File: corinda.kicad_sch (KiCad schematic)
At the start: 15 parts, among them J1 Pixels, J2 USB_B_Micro, J3 ExtPwr, J4 ExtPwr2, SW1 RESET, U1 ME6211, U2 ESP-C3-13U, U3 D1_Mini_16p

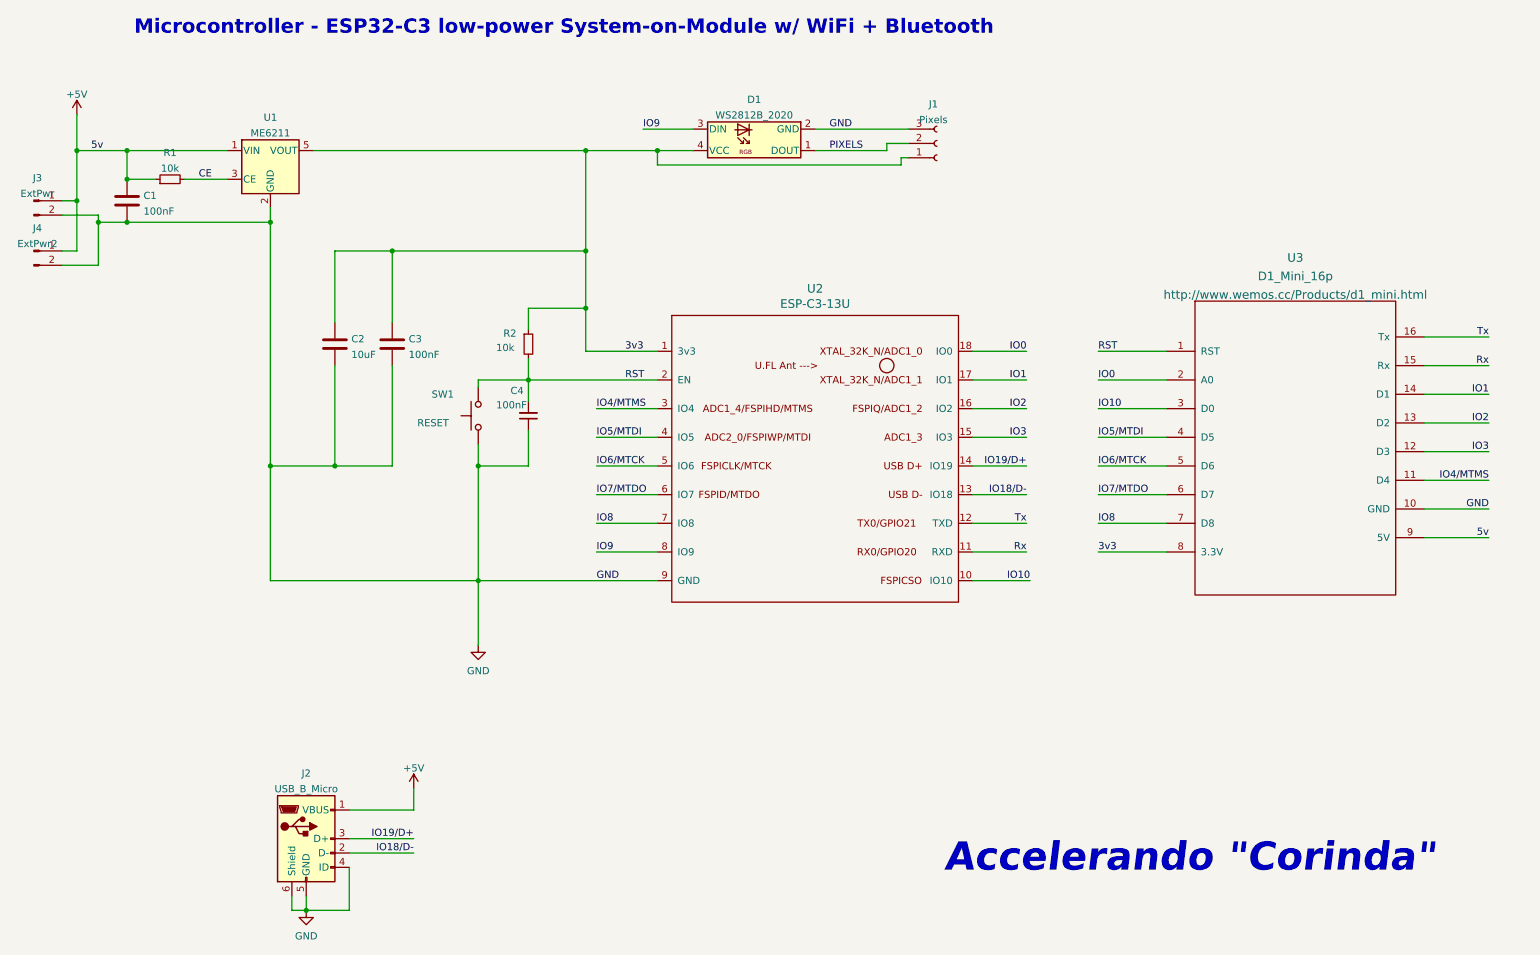
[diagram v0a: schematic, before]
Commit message: Corinda 1v1
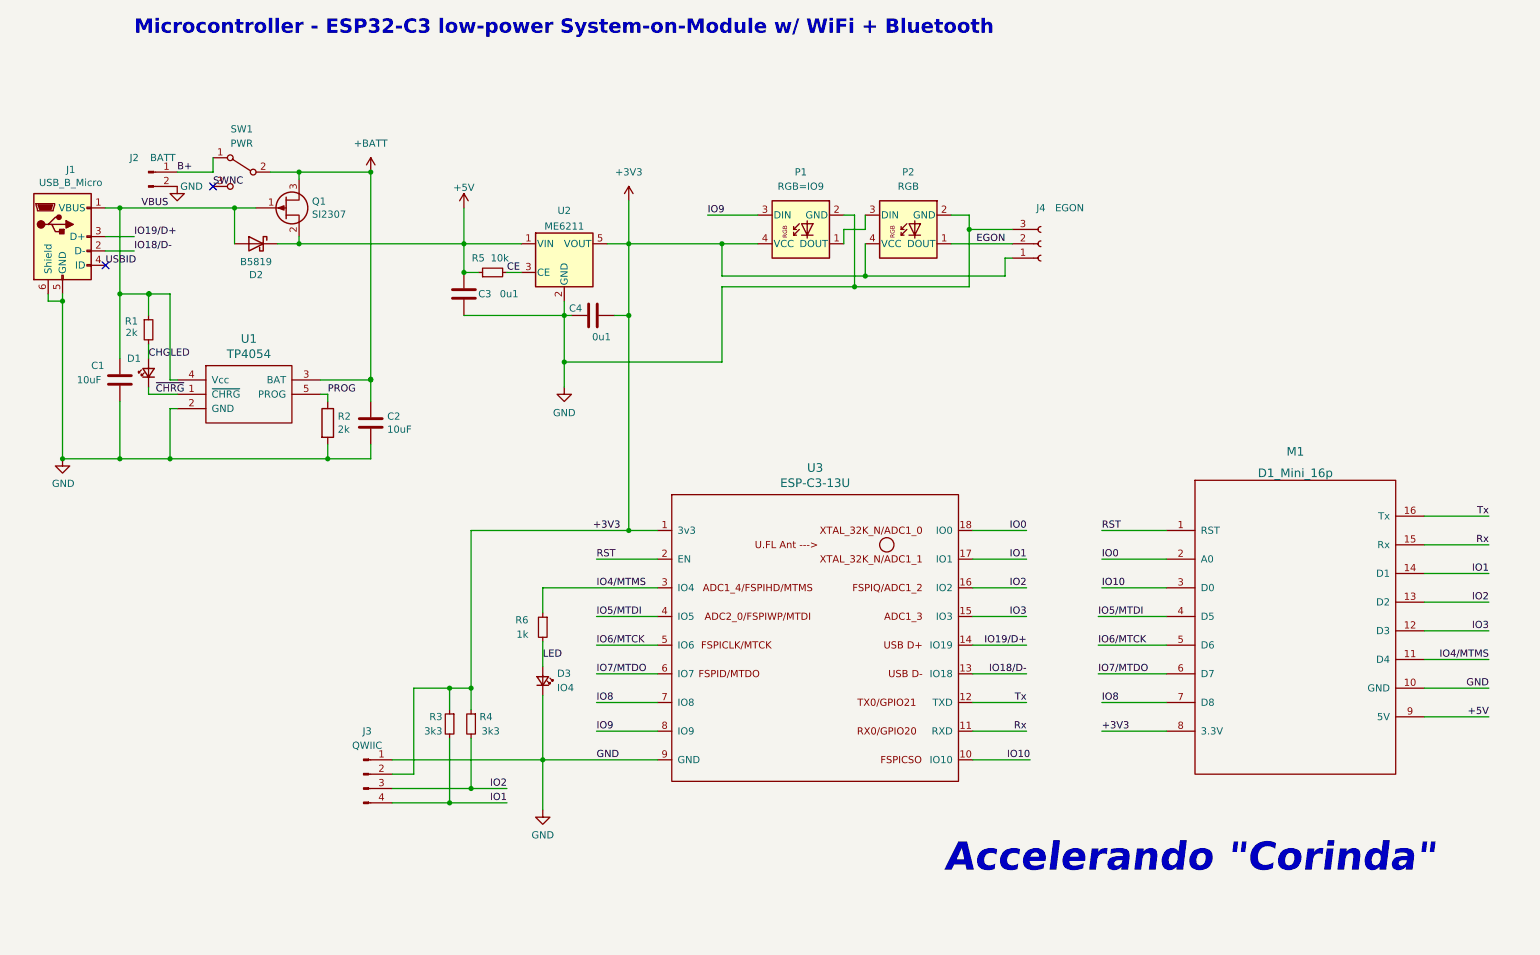
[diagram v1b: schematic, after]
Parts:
- removed C3: 100nF, Capacitor_SMD:C_0603_1608Metric_Pad1.08x0.95mm_HandSolder, symbol Device:C
- removed C4: 100nF, Capacitor_SMD:C_0603_1608Metric_Pad1.08x0.95mm_HandSolder, symbol Device:C_Small
- removed D1: WS2812B_2020, Accelerando:LED_WS2812B_PLCC2_0x1_8mm_P1.27mm, symbol Accelerando:WS2812B_2020
- removed J2: USB_B_Micro, Accelerando:USB_Micro_SMD, symbol Connector:USB_B_Micro
- removed J3: ExtPwr, Connector_JST:JST_GH_SM02B-GHS-TB_1x02-1MP_P1.25mm_Horizontal, symbol Connector:Conn_01x02_Male
- removed J4: ExtPwr2, Connector_PinHeader_1.27mm:PinHeader_1x02_P1.27mm_Vertical, symbol Connector:Conn_01x02_Male
- removed R2: 10k, Resistor_SMD:R_0603_1608Metric_Pad0.98x0.95mm_HandSolder, symbol Device:R_Small
- removed SW1: RESET, Accelerando:TVBM02, symbol Switch:SW_Push
- added C1: 10uF, Capacitor_SMD:C_0402_1005Metric, symbol Device:C
- added C4: 0u1, Capacitor_SMD:C_0402_1005Metric, symbol Device:C
- added D1: CHG, LED_SMD:LED_0402_1005Metric, symbol Device:LED_Small
- added D2: B5819, Diode_SMD:D_SOD-123, symbol Device:D_Schottky
- added D3: IO4, LED_SMD:LED_0402_1005Metric, symbol Device:LED_Small
- added J1: USB_B_Micro, Accelerando:USB_Micro_SMD, symbol accelerando_hailstone-rescue:USB_B_Micro-Connector
- added J2: BATT, Connector_JST:JST_GH_SM02B-GHS-TB_1x02-1MP_P1.25mm_Horizontal, symbol Connector:Conn_01x02_Male
- added J3: QWIIC, Connector_JST:JST_SH_SM04B-SRSS-TB_1x04-1MP_P1.00mm_Horizontal, symbol Connector:Conn_01x04_Male
- added P1: RGB=IO9, Accelerando:LED_WS2812B_PLCC2_0x1_8mm_P1.27mm, symbol Accelerando:WS2812B_2020
- added P2: RGB, Accelerando:LED_WS2812B_PLCC2_0x1_8mm_P1.27mm, symbol Accelerando:WS2812B_2020
- added Q1: SI2307, Package_TO_SOT_SMD:SOT-23, symbol Device:Q_PJFET_GSD
- added R1: 2k, Resistor_SMD:R_0402_1005Metric, symbol Device:R_Small
- added R2: 2k, Resistor_SMD:R_0402_1005Metric, symbol Device:R
- added R3, R4: 3k3, Resistor_SMD:R_0402_1005Metric, symbol Device:R_Small
- added R6: 1k, Resistor_SMD:R_0402_1005Metric, symbol Device:R_Small
- added SW1: PWR, Button_Switch_SMD:SW_SPDT_PCM12, symbol Switch:SW_SPDT
- added U1: TP4054, Package_TO_SOT_SMD:SOT-23-5, symbol Accelerando:TP4054
- C2: footprint Capacitor_SMD:C_0805_2012Metric_Pad1.18x1.45mm_HandSolder -> Capacitor_SMD:C_0402_1005Metric
- C3: renamed from C1; value 100nF -> 0u1; footprint Capacitor_SMD:C_0603_1608Metric_Pad1.08x0.95mm_HandSolder -> Capacitor_SMD:C_0402_1005Metric
- J4: renamed from J1; value Pixels -> EGON; footprint Connector_JST:JST_XH_S3B-XH-A_1x03_P2.50mm_Horizontal -> Connector_JST:JST_GH_SM03B-GHS-TB_1x03-1MP_P1.25mm_Horizontal
- R5: renamed from R1; footprint Resistor_SMD:R_0603_1608Metric_Pad0.98x0.95mm_HandSolder -> Resistor_SMD:R_0402_1005Metric
- renumbered U3 to M1, U1 to U2, U2 to U3
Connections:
- net +5V: now also D2.1 (K), Q1.2 (S)
- net GND: now also C1.2, C4.1, D3.1 (K), J1.5 (GND), J1.6 (Shield), J2.2 (Pin_2), J3.1 (Pin_1), P1.2 (GND), P2.2 (GND), R2.2, U1.2 (GND)
- net IO1: now also J3.4 (Pin_4), R3.2
- net IO18/D-: now also J1.2 (D-)
- net IO19/D+: now also J1.3 (D+)
- net IO2: now also J3.3 (Pin_3), R4.2
- net IO4/MTMS: now also R6.1
- net IO9: now also P1.3 (DIN)
- net 3v3 renamed +3V3
- net +3V3: now also C4.2, J3.2 (Pin_2), P1.4 (VCC), P2.4 (VCC), R3.1, R4.1; no longer C2.1
- net PIXELS renamed EGON
- net EGON: now also P2.1 (DOUT)
- new net: P1.1 (DOUT), P2.3 (DIN)
- new net +BATT: C2.1, Q1.3 (D), SW1.2 (B), U1.3 (BAT)
- new net B+: J2.1 (Pin_1), SW1.1 (A)
- new net CHGLED: D1.2 (A), R1.2
- new net LED: D3.2 (A), R6.2
- new net PROG: R2.1, U1.5 (PROG)
- new net SWNC: SW1.3 (C)
- new net USBID: J1.4 (ID)
- new net VBUS: C1.1, D2.2 (A), J1.1 (VBUS), Q1.1 (G), R1.1, U1.4 (Vcc)
- new net ~{CHRG}: D1.1 (K), U1.1 (~{CHRG})
- no-connect marks 0 -> 2
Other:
- moved on the sheet: C3, J4, M1, R5, U2, U3
